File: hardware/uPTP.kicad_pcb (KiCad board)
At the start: 2 copper layers, 33 x 30 mm, 5 parts, among them U1 CH32V307WCU6, U2 HC-RJ45-055-7

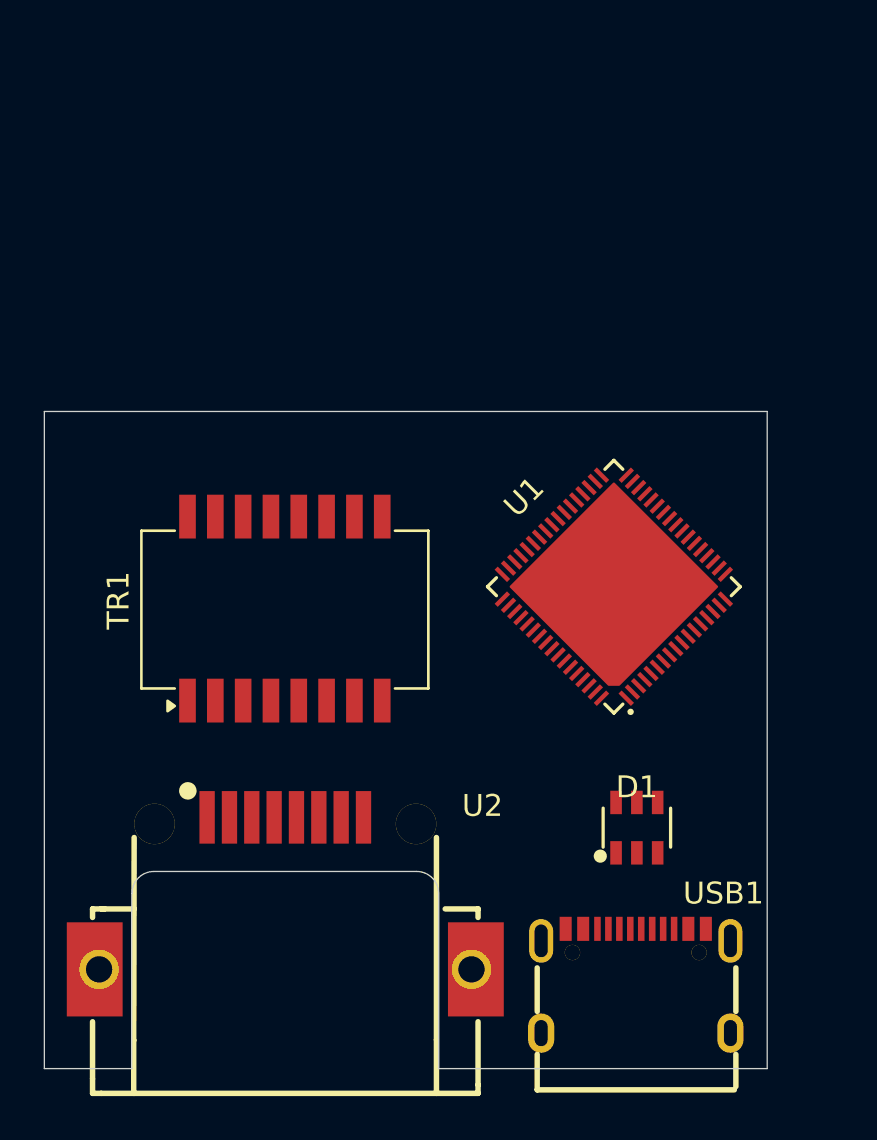
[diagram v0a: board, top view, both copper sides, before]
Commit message: Nice first render
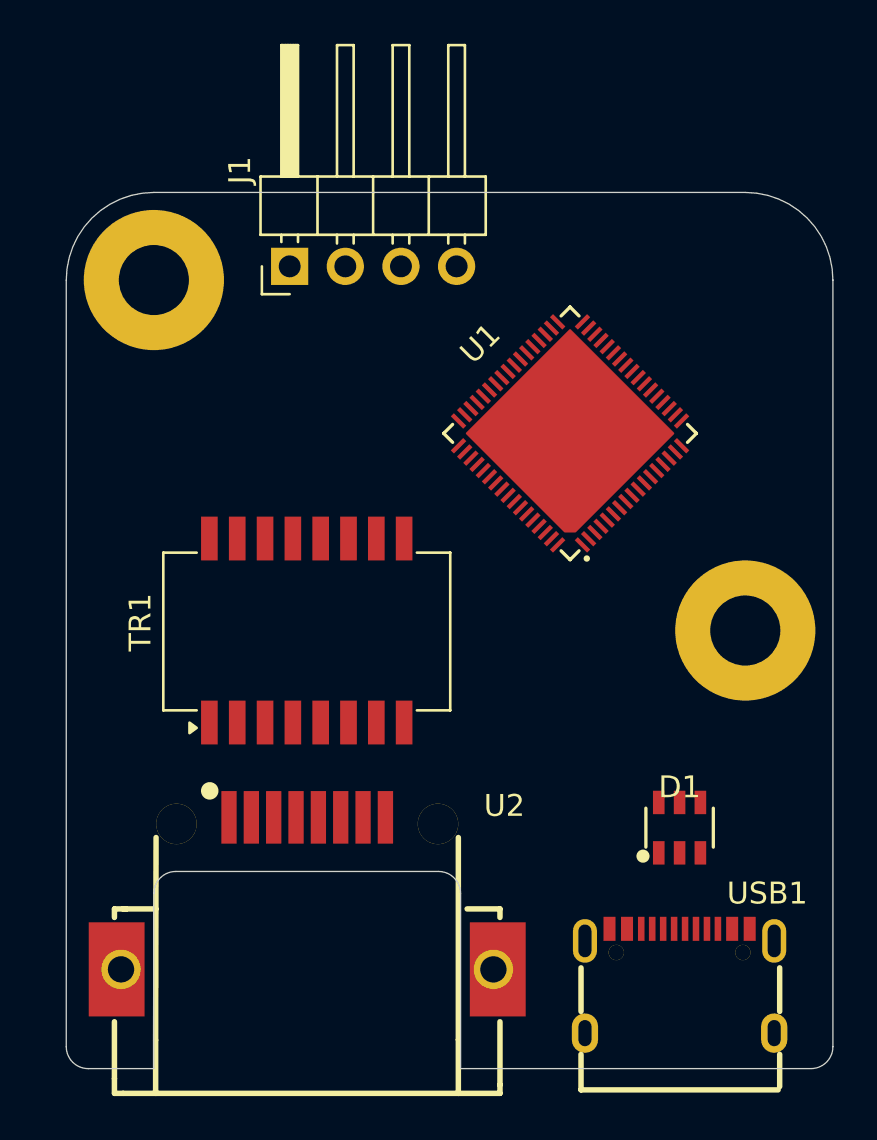
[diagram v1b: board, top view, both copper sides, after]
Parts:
- added H1: MountingHole_Pad, MountingHole:MountingHole_3.2mm_M3_Pad, F.Cu at (161.0, 110.0)
- added H2: MountingHole_Pad, MountingHole:MountingHole_3.2mm_M3_Pad, F.Cu at (134.0, 94.0)
- added J1: Conn_01x04_Pin, Connector_PinHeader_2.54mm:PinHeader_1x04_P2.54mm_Horizontal, F.Cu at (140.2, 93.4)
- moved U1 7.28 mm to (153.0, 101.0)
- moved USB1 2.00 mm to (158.0, 126.0)
- moved D1 1.95 mm to (158.0, 119.0)
- moved TR1 1.41 mm to (141.0, 110.0)
- moved U2 1.00 mm to (141.0, 122.0)
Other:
- board size 33 x 30 mm -> 35 x 40 mm
